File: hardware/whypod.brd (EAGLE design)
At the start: 72.1 x 85.1 mm, 30 parts, among them IC1 IC_USBLC6-2, J1 AUDIO_JACK_TRRSSMD_RA, U1 USD-SOCKETUSD, X2 USB-A-S, Y1 CRYSTAL-GROUNDEDSMD-5X3.2

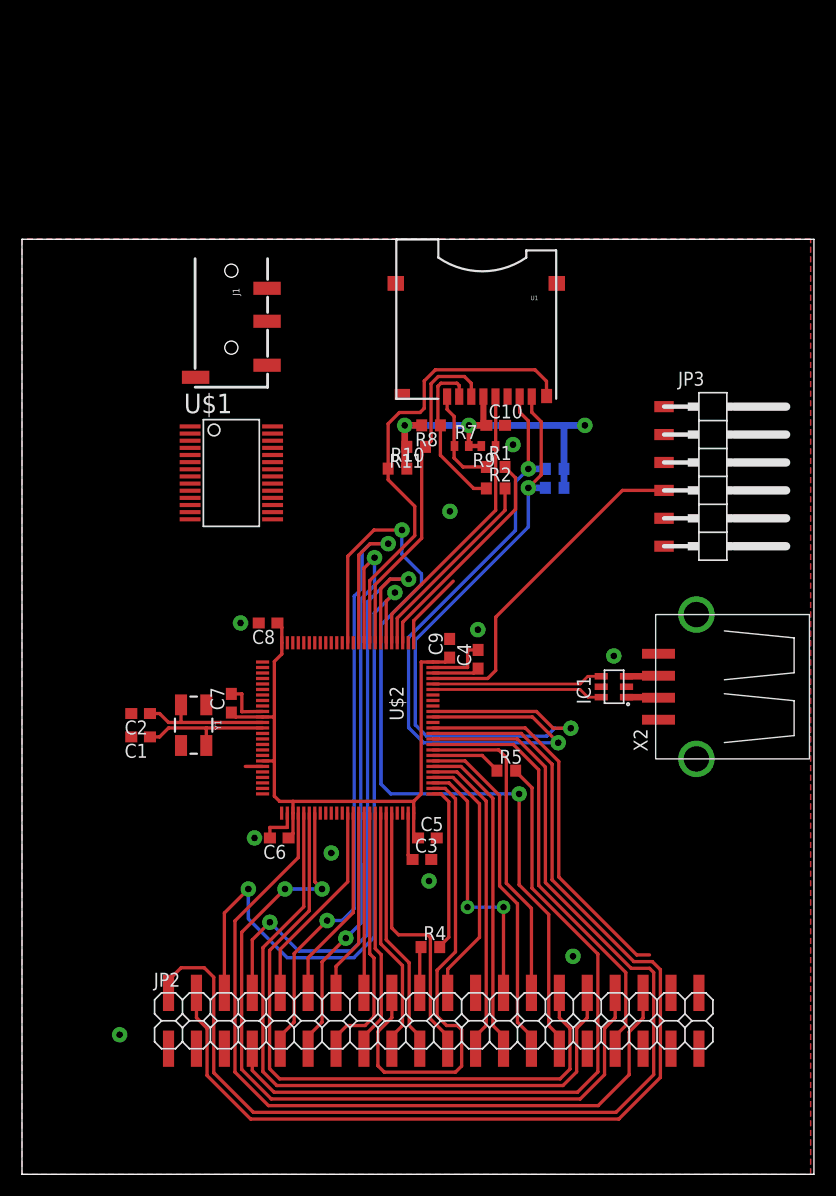
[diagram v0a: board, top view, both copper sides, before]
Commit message: PCB updates
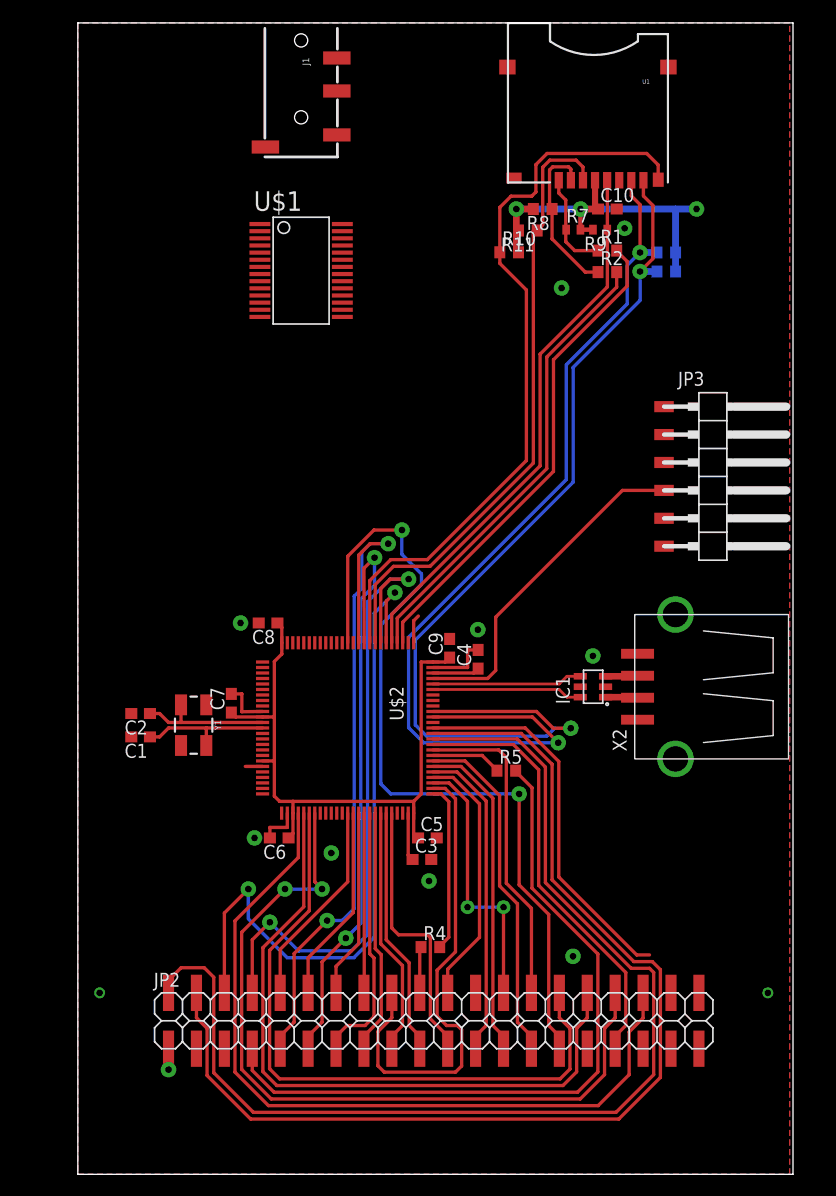
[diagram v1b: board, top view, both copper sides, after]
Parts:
- moved C10 22.2 mm to (53.3, 87.8)
- moved R6 22.2 mm to (58.6, 82.1)
- moved U1 22.2 mm to (52.0, 104.7)
- moved R3 22.2 mm to (58.6, 83.9)
- moved R8 22.2 mm to (47.4, 87.8)
- moved R2 22.2 mm to (53.3, 82.1)
- moved R1 22.2 mm to (53.3, 84.0)
- moved R11 22.2 mm to (46.0, 85.9)
- moved R9 22.2 mm to (52.6, 86.0)
- moved R10 22.2 mm to (44.3, 83.9)
- moved R7 22.2 mm to (50.2, 86.0)
- moved J1 21.9 mm to (25.4, 104.8)
- moved U$1 19.5 mm to (25.4, 81.9)
- moved IC1 1.91 mm to (50.8, 44.4)
- moved X2 1.91 mm to (59.5, 44.4)
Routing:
- net SDIO_CMD: track 31.6 -> 57.5 mm
- net SDIO_CD: track 42.5 -> 68.3 mm
- net SDIO_D1: track 64.5 -> 88.4 mm
- net SDIO_CLK: track 26.6 -> 50.5 mm
- net N$8: track 18.1 -> 42.0 mm
- net SDIO_D0: track 63.1 -> 87.0 mm
- net N$5: track 21.2 -> 45.1 mm
- net SWD_CLK: track 7.10 -> 2.61 mm
- net USB_D_P: track 15.6 -> 13.7 mm
- net USB_D_N: track 15.6 -> 13.7 mm
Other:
- board size 72.1 x 85.1 mm -> 65.1 x 104.8 mm
